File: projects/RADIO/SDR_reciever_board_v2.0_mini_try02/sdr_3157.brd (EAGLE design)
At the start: 70 x 75 mm, 55 parts, among them IC1 LM1117-33, IC2 L7805CV, U1 NE5532D, U2 SN74LVC1G3157DBVR, U3 SN74LVC1G3157DBVR

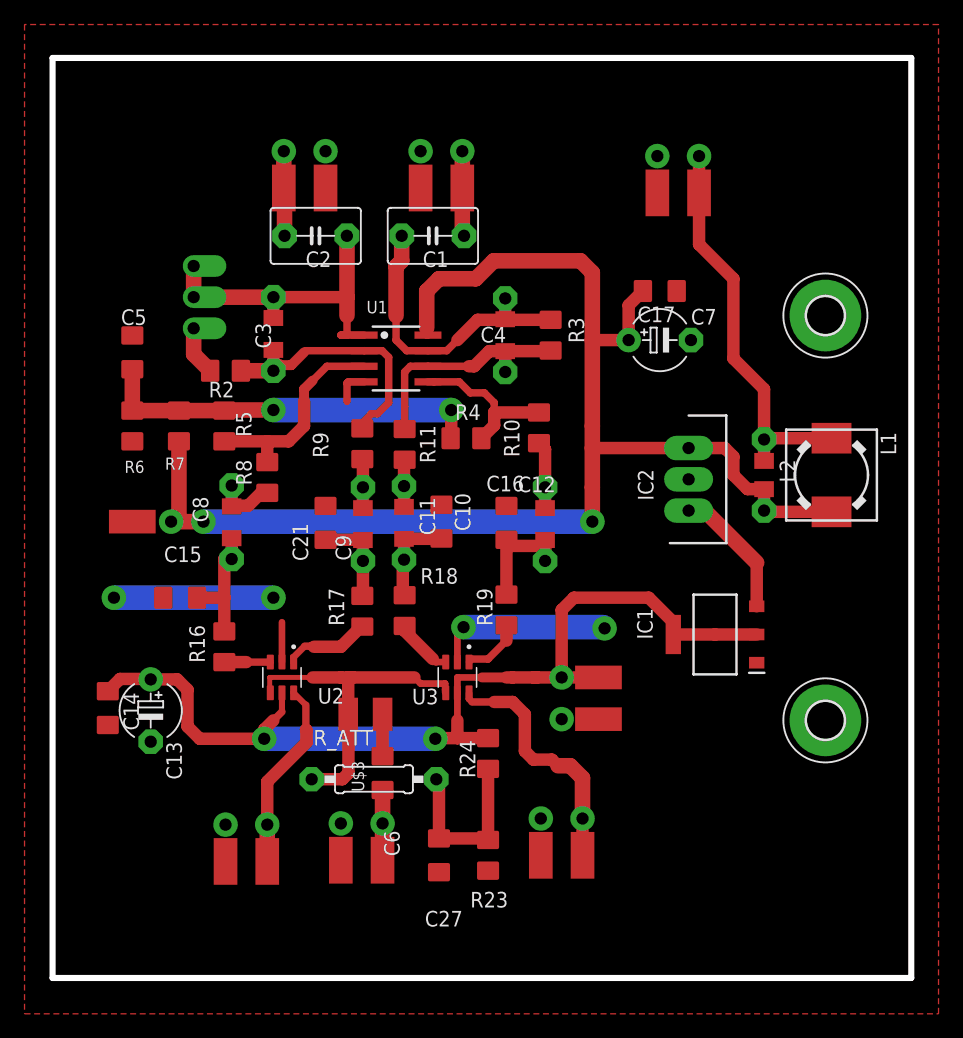
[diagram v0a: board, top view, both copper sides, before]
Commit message: Update
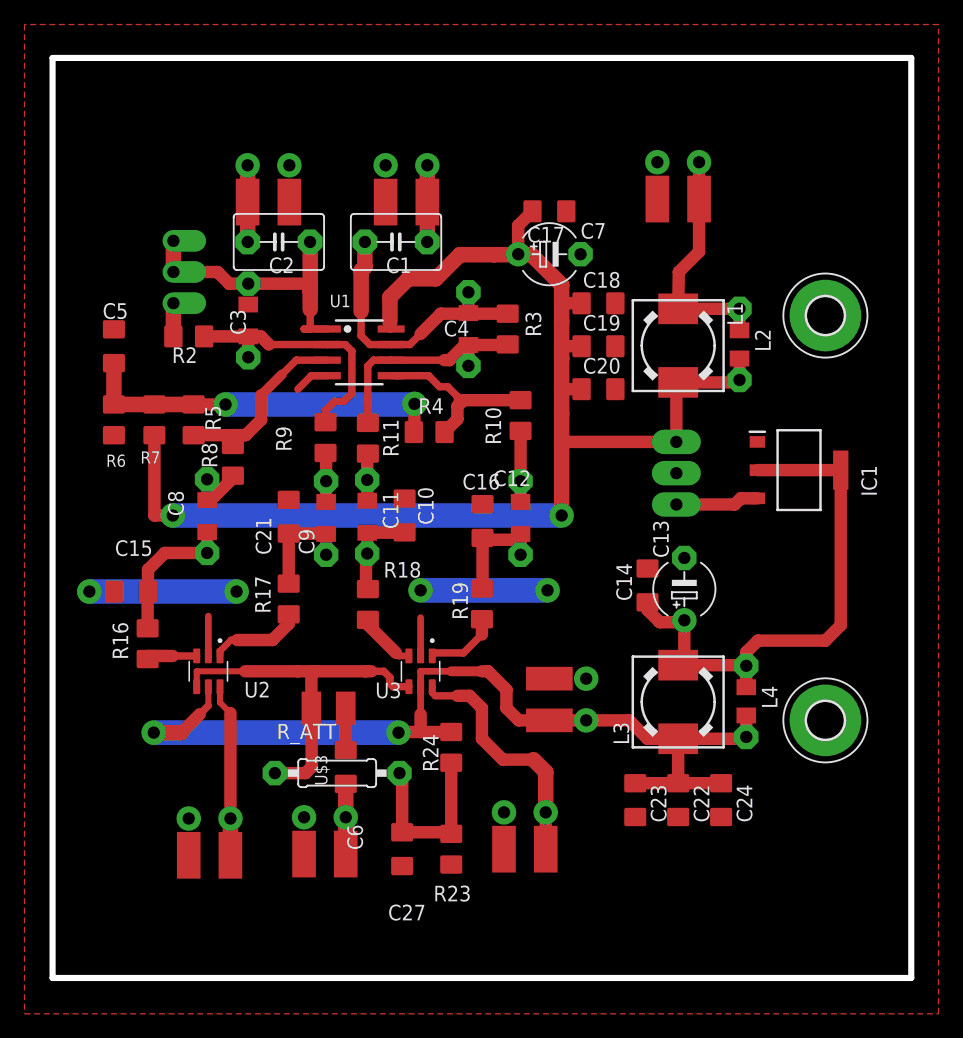
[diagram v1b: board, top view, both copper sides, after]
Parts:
- removed P_1: SMD_PTH_PIN, mylib:SMD_PTH_PIN
- added C18, C19, C20, C22, C23, C24: (no value), mylib:C0805
- added L3: DR74, inductors:DR74
- added L4: (no value), mylib:M0805
- moved C14 45.1 mm to (48.5, 32.0), turned to 90 degrees
- moved C13 44.6 mm to (51.5, 31.7), turned to 90 degrees
- moved L1 16.4 mm to (51.0, 51.5)
- moved IC1 15.0 mm to (60.9, 41.4), turned to 0 degrees
- moved C7 11.4 mm to (40.5, 59.0)
- moved C17 11.1 mm to (40.5, 62.5)
- moved L2 10.8 mm to (56.0, 51.6)
- moved R16 6.25 mm to (7.75, 27.2)
- moved R17 6.08 mm to (19.2, 30.9)
- moved U2 6.02 mm to (12.7, 25.0)
- moved R2 4.10 mm to (11.1, 52.3)
- moved C15 4.03 mm to (6.40, 31.5)
- moved 3V3 4.00 mm to (40.5, 22.7), turned to 0 degrees
- moved R3 3.54 mm to (37.1, 52.9)
- moved Q 3.17 mm to (17.6, 63.2)
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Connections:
- new net N$6: C13.+, C14.1, IC1.2, IC1.4, L3.2, L4.1, L4.P$1
- net 12V: now also C18.1, C19.1, C20.1; no longer P_1.P$1, P_1.P$2
- net GND: now also C18.2, C19.2, C20.2, C22.2, C23.2, C24.2
- net VCC: now also C22.1, C23.1, C24.1, L3.1, L4.2, L4.P$2; no longer C13.+, C14.1, IC1.2, IC1.4
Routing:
- net N$6: track 0.00 -> 44.5 mm
- net VIN: track 32.6 -> 19.4 mm
- net 5V: track 10.9 -> 6.81 mm
- net N$21: track 27.2 -> 23.6 mm
- net ANTENNA: track 27.6 -> 30.9 mm
- net 12V: track 110.6 -> 107.6 mm
- net GND: track 33.8 -> 31.6 mm
- net N$18: track 13.1 -> 14.8 mm
- net N$24: track 24.5 -> 22.9 mm
- net N$20: track 31.8 -> 30.3 mm
- net N$8: track 10.4 -> 11.9 mm
- net COS_IN: track 15.5 -> 14.1 mm
- net VCC: track 79.7 -> 78.3 mm
- net N$28: track 4.02 -> 2.71 mm
- net N$9: track 7.63 -> 8.83 mm
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
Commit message: Update
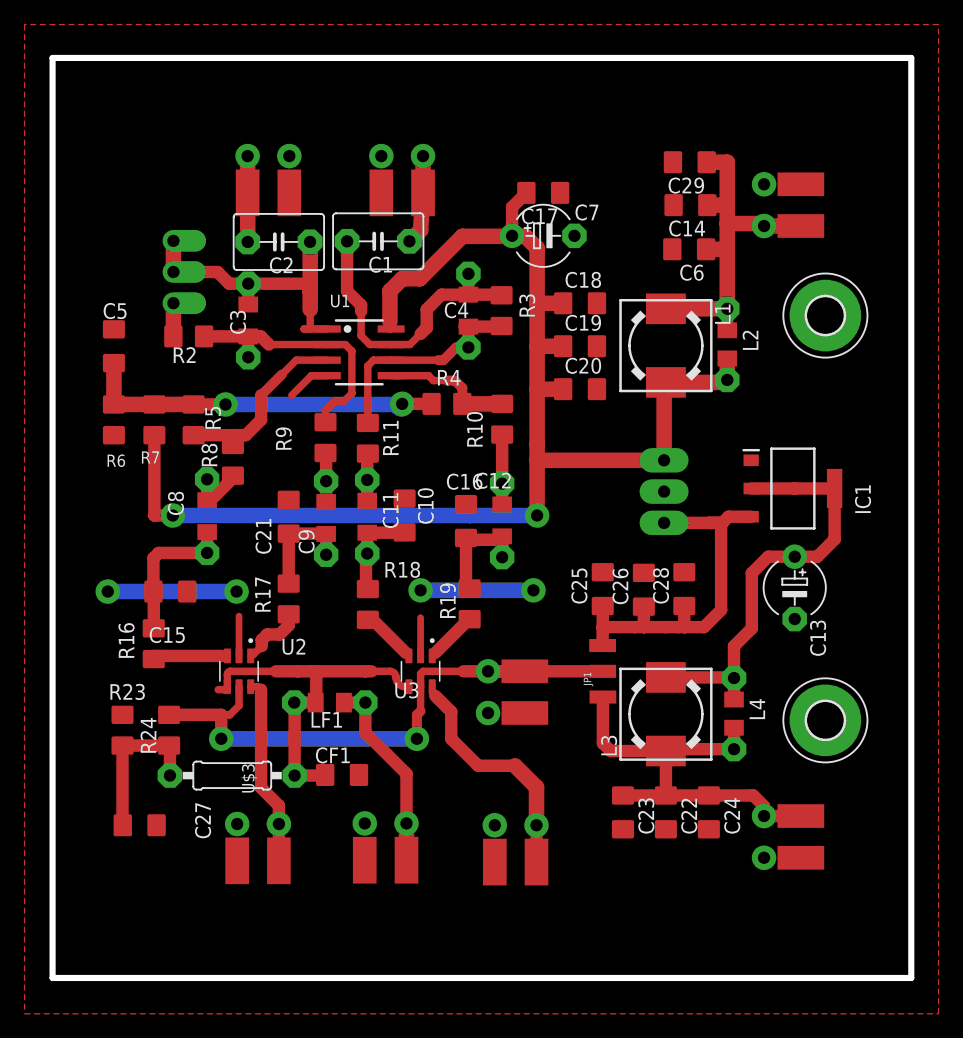
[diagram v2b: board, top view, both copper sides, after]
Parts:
- removed RF_IN1: 2X_SMD_PTH_PIN, mylib:2X_SMD_PTH
- removed R_ATT: 20, rcl:R1210
- added C25, C26, C28, C29: (no value), mylib:C0805
- added CF1: 22nF, mylib:C0805
- added JP1: JUMPER-SMT_3_1-NC_PASTE_NO-SILK, SparkFun-Jumpers:SMT-JUMPER_3_1-NC_PASTE_NO-SILK
- added LF1: 20, mylib:M0805
- added MC_3V3, VIN: 2X_SMD_PTH_PIN, mylib:2X_SMD_PTH
- C6: value 22nF -> (none)
- moved C6 50.6 mm to (51.9, 59.4), turned to 180 degrees
- moved C14 31.2 mm to (52.0, 63.0), turned to 180 degrees
- moved R23 28.5 mm to (5.70, 20.2), turned to 270 degrees
- moved R24 23.0 mm to (9.50, 20.2)
- moved C27 21.5 mm to (7.10, 12.4), turned to 180 degrees
- moved C13 9.00 mm to (60.5, 31.8), turned to 270 degrees
- moved U$3 8.55 mm to (14.7, 16.5), turned to 0 degrees
- moved RF_IN 4.98 mm to (27.1, 9.60)
- moved COS 3.98 mm to (16.8, 9.55)
- moved C15 3.20 mm to (9.60, 31.5), turned to 0 degrees
- moved R4 2.72 mm to (32.1, 46.8)
- moved U2 2.50 mm to (15.2, 25.0)
- moved 3V3 2.09 mm to (38.5, 23.3), turned to 180 degrees
- moved IC2 1.80 mm to (49.9, 42.2)
- moved C17 1.58 mm to (40.0, 64.0)
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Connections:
- removed net N$2: C6.1, R_ATT.1
- new net 3.3V: C22.1, C23.1, C24.1, JP1.1, L3.1, L4.2, L4.P$2, MC_3V3.P$2, MC_3V3.T$2
- net 5V: now also C25.1, C26.1, C28.1, JP1.3
- net ANTENNA: now also CF1.2, LF1.2, LF1.P$2; no longer R_ATT.2
- net GND: now also C25.2, C26.2, C28.2, C29.2, C6.2, CF1.1, MC_3V3.P$1, MC_3V3.T$1, VIN.P$2, VIN.T$2; no longer RF_IN1.P$1, RF_IN1.T$1
- net N$1: now also LF1.1, LF1.P$1; no longer C6.2
- net N$6: no longer C14.1
- net VCC: now also JP1.2; no longer C22.1, C23.1, C24.1, L3.1, L4.2, L4.P$2
- net VIN: now also C14.1, C29.1, C6.1, VIN.P$1, VIN.T$1; no longer RF_IN1.P$2, RF_IN1.T$2
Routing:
- net 3.3V: track 0.00 -> 35.8 mm
- net VCC: track 78.3 -> 48.8 mm
- net 5V: track 6.81 -> 32.3 mm
- net VIN: track 19.4 -> 29.8 mm
- net N$1: track 5.72 -> 16.0 mm
- net N$6: track 44.5 -> 35.3 mm
- net N$18: track 14.8 -> 10.8 mm
- net 12V: track 107.6 -> 111.2 mm
- net N$2: track 3.42 -> 0.00 mm
- net N$4: track 7.69 -> 5.36 mm
- net N$25: track 14.9 -> 12.8 mm
- net N$3: track 4.25 -> 6.25 mm
- net GND: track 31.6 -> 29.6 mm
- net N$7: track 6.02 -> 4.29 mm
- net N$21: track 23.6 -> 25.3 mm
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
